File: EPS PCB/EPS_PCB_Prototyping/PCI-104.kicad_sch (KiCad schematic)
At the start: 6 parts, among them J1 Conn_02x32_Row_Letter_First, J2 Conn_02x20_Row_Letter_First

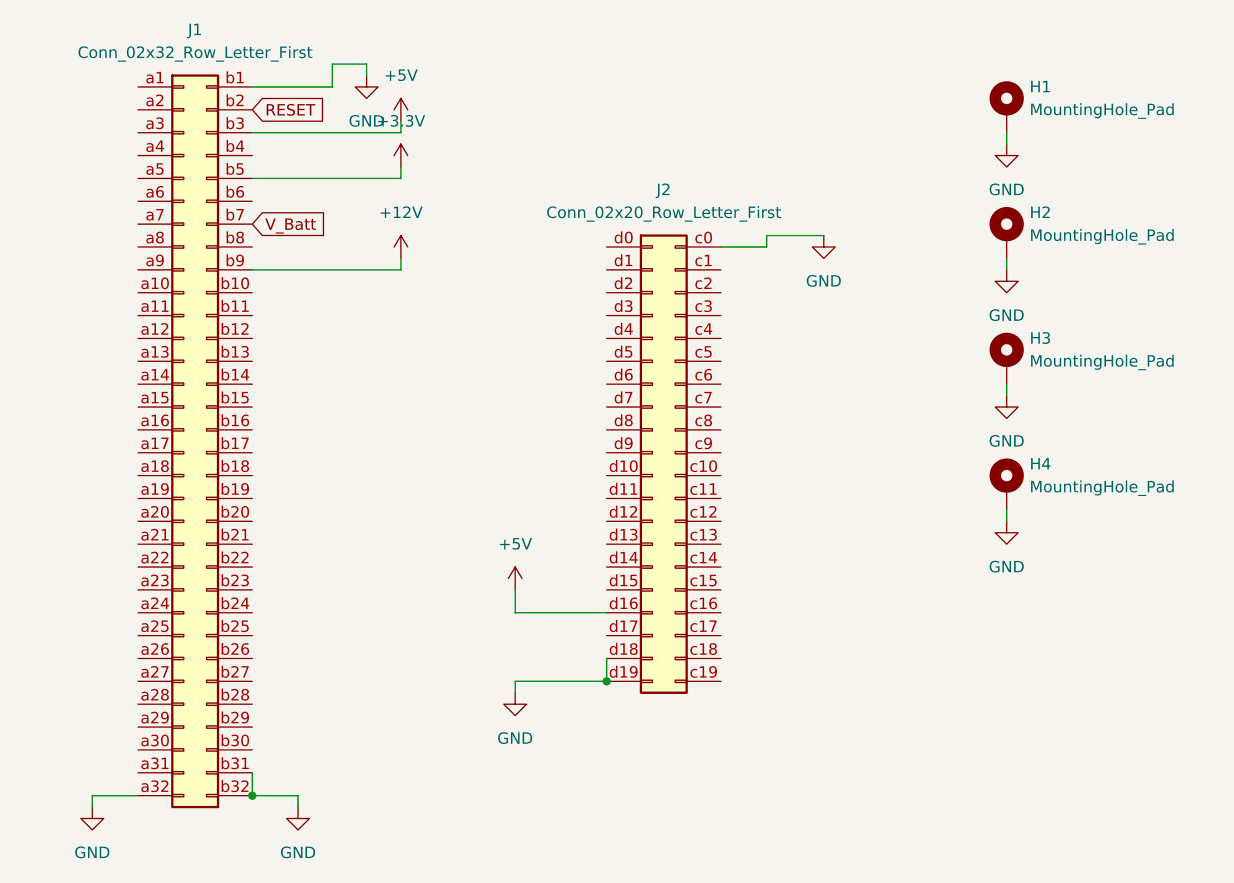
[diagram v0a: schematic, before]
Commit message: Prototype board v1 finished
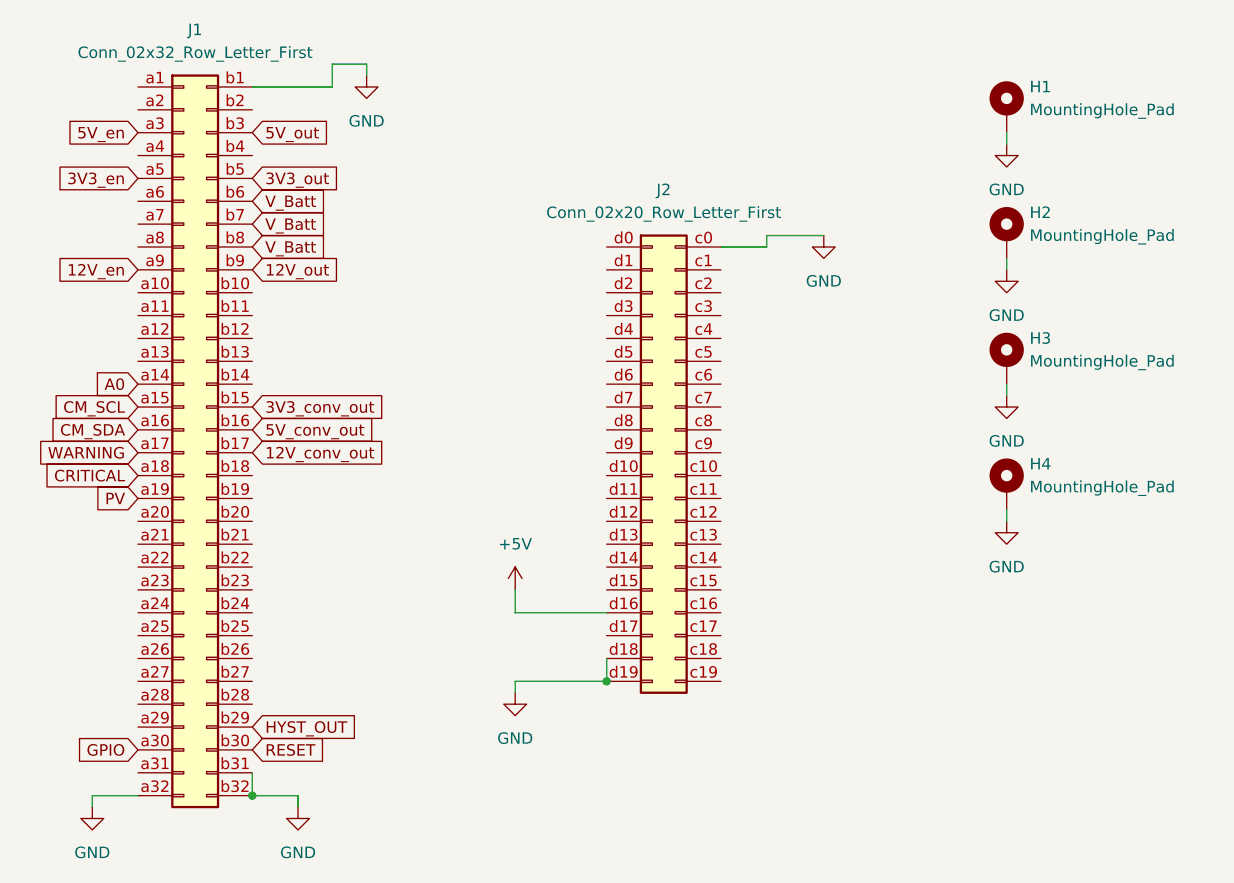
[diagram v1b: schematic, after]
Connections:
- net +5V: no longer J1.b3 (Pin_b3)
- net RESET: now also J1.b30 (Pin_b30); no longer J1.b2 (Pin_b2)
- net V_Batt: now also J1.b6 (Pin_b6), J1.b8 (Pin_b8)
- net A0: now reaches J1.a14 (Pin_a14)
- net CM_SCL: now reaches J1.a15 (Pin_a15)
- net CM_SDA: now reaches J1.a16 (Pin_a16)
- net WARNING: now reaches J1.a17 (Pin_a17)
- net CRITICAL: now reaches J1.a18 (Pin_a18)
- net PV: now reaches J1.a19 (Pin_a19)
- net 5V_en: now reaches J1.a3 (Pin_a3)
- net GPIO: now reaches J1.a30 (Pin_a30)
- net 3V3_en: now reaches J1.a5 (Pin_a5)
- net 12V_en: now reaches J1.a9 (Pin_a9)
- net 3V3_conv_out: now reaches J1.b15 (Pin_b15)
- net 5V_conv_out: now reaches J1.b16 (Pin_b16)
- net 12V_conv_out: now reaches J1.b17 (Pin_b17)
- net HYST_OUT: now reaches J1.b29 (Pin_b29)
- net +12V renamed 12V_out
- net +3.3V renamed 3V3_out
- new net 5V_out: J1.b3 (Pin_b3)
